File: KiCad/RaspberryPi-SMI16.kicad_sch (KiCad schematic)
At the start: 11 parts, among them J1 Screw_Terminal_01x02, U1 RASPBERRYPI_GPIO_40, U2 RFID-RC522

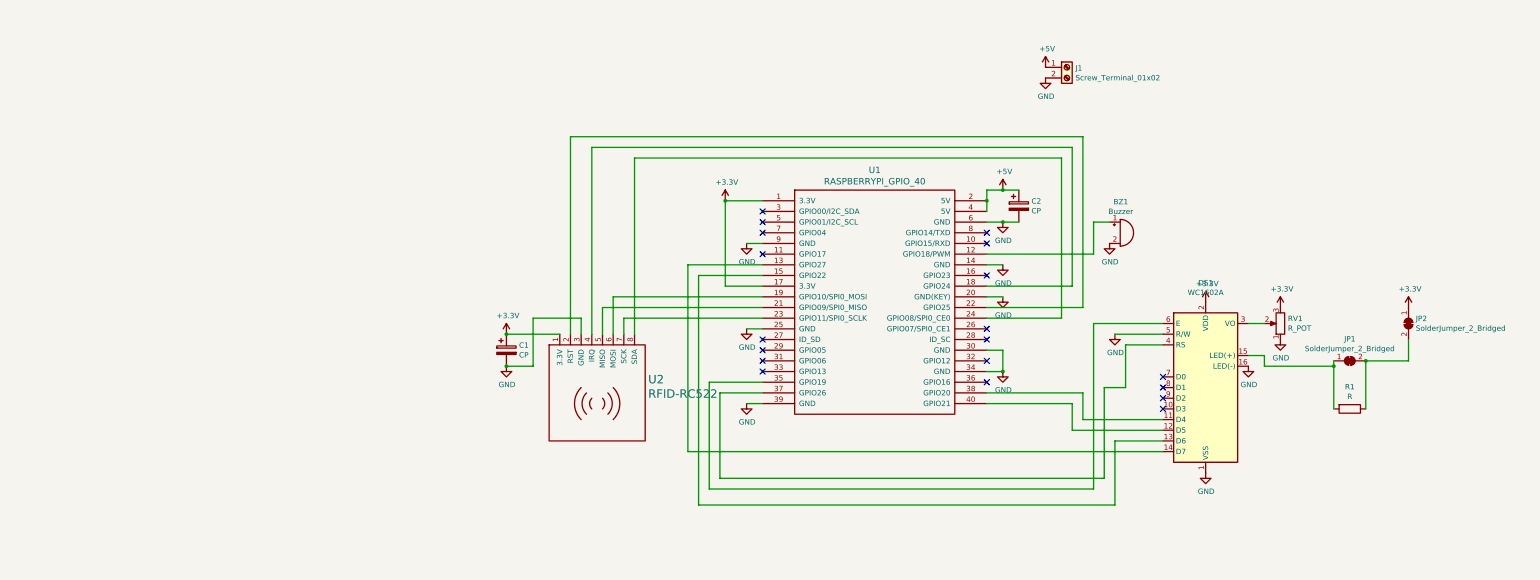
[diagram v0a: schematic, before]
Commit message: SMI HAT PCB create
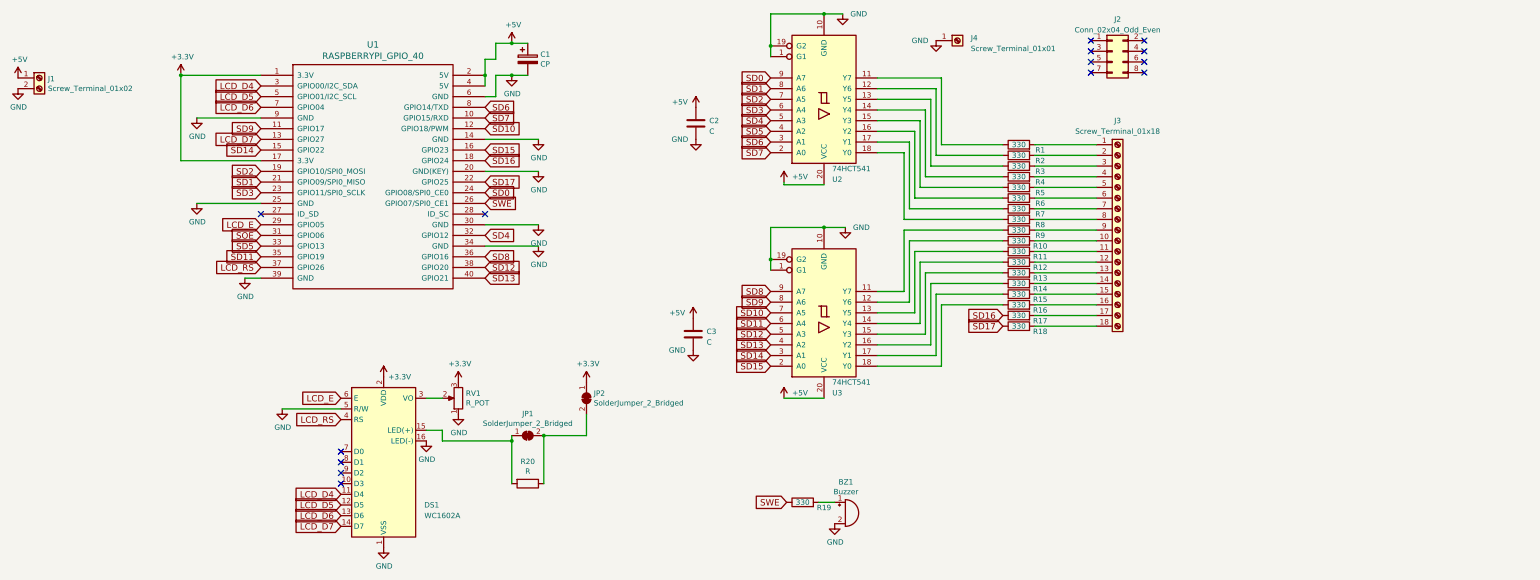
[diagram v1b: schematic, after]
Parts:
- removed C1: CP, Capacitor_THT:CP_Radial_D8.0mm_P3.50mm, symbol RaspberryPi-SMI16-rescue:CP-Device
- removed U2: RFID-RC522, library:RFID-RC522, symbol RaspberryPi-SMI16-rescue:RFID-RC522-nanbuwks
- added C2, C3: C, Capacitor_SMD:C_0603_1608Metric, symbol Device:C
- added J2: Conn_02x04_Odd_Even, MountingHole:MountingHole_3.2mm_M3, symbol Connector_Generic:Conn_02x04_Odd_Even
- added J3: Screw_Terminal_01x18, Connector_PinHeader_2.54mm:PinHeader_1x18_P2.54mm_Vertical, symbol Connector:Screw_Terminal_01x18
- added J4: Screw_Terminal_01x01, Connector_PinHeader_2.54mm:PinHeader_1x01_P2.54mm_Vertical, symbol Connector:Screw_Terminal_01x01
- added R1, R10, R11, R12, R13, R14, R15, R16, R17, R18, R19, R2, R3, R4, R5, R6, R7, R8, R9: 330, Resistor_SMD:R_0603_1608Metric, symbol Device:R
- added U2: 74HCT541, Package_SO:SOIC-20W_7.5x12.8mm_P1.27mm, symbol 74xx:74HCT541
- added U3: 74HCT541, Package_SO:SOIC-20W_7.5x15.4mm_P1.27mm, symbol 74xx:74HCT541
- J1: footprint TerminalBlock:TerminalBlock_bornier-2_P5.08mm -> TerminalBlock_Phoenix:TerminalBlock_Phoenix_MKDS-1,5-2_1x02_P5.00mm_Horizontal
- renumbered C2 to C1, R1 to R20
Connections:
- net +5V: now also C2.1, C3.1, U2.20 (VCC), U3.20 (VCC)
- net GND: now also C2.2, C3.2, J4.1 (Pin_1), U2.1 (G1), U2.10 (GND), U2.19 (G2), U3.1 (G1), U3.10 (GND), U3.19 (G2)
- net SD17: now reaches U1.22 (GPIO25)
- net SD17: now also R18.1
- net SD16: now reaches U1.18 (GPIO24)
- net SD16: now also R17.1
- net SD1: now reaches U1.21 (GPIO09/SPI0_MISO)
- net SD1: now also U2.8 (A6)
- net SD2: now reaches U1.19 (GPIO10/SPI0_MOSI)
- net SD2: now also U2.7 (A5)
- net SD3: now reaches U1.23 (GPIO11/SPI0_SCLK)
- net SD3: now also U2.6 (A4)
- net SD0: now reaches U1.24 (GPIO08/SPI0_CE0)
- net SD0: now also U2.9 (A7)
- net LCD_D4: now reaches DS1.11 (D4)
- net LCD_D4: now also U1.3 (GPIO00/I2C_SDA); no longer U1.38 (GPIO20)
- net LCD_D5: now reaches DS1.12 (D5)
- net LCD_D5: now also U1.5 (GPIO01/I2C_SCL); no longer U1.40 (GPIO21)
- net LCD_D6: now reaches DS1.13 (D6)
- net LCD_D6: now also U1.7 (GPIO04); no longer U1.15 (GPIO22)
- net LCD_D7: now reaches DS1.14 (D7), U1.13 (GPIO27)
- net LCD_RS: now reaches DS1.4 (RS), U1.37 (GPIO26)
- net LCD_E: now reaches DS1.6 (E)
- net LCD_E: now also U1.29 (GPIO05); no longer U1.35 (GPIO19)
- net at BZ1.1 (-): now also R19.2; no longer U1.12 (GPIO18/PWM)
- net SD7: now reaches U1.10 (GPIO15/RXD)
- net SD7: now also U2.2 (A0)
- net SD9: now reaches U1.11 (GPIO17)
- net SD9: now also U3.8 (A6)
- net SD15: now reaches U1.16 (GPIO23)
- net SD15: now also U3.2 (A0)
- net SWE: now reaches U1.26 (GPIO07/SPI0_CE1)
- net SWE: now also R19.1
- net SOE: now reaches U1.31 (GPIO06)
- net SD4: now reaches U1.32 (GPIO12)
- net SD4: now also U2.5 (A3)
- net SD5: now reaches U1.33 (GPIO13)
- net SD5: now also U2.4 (A2)
- net SD8: now reaches U1.36 (GPIO16)
- net SD8: now also U3.9 (A7)
- net SD6: now reaches U1.8 (GPIO14/TXD)
- net SD6: now also U2.3 (A1)
- new net: R16.1, U3.18 (Y0)
- new net: J3.16 (Pin_16), R16.2
- new net: R14.1, U3.16 (Y2)
- new net: J3.14 (Pin_14), R14.2
- new net: J3.17 (Pin_17), R17.2
- new net: R4.1, U2.14 (Y4)
- new net: J3.4 (Pin_4), R4.2
- new net: R6.1, U2.16 (Y2)
- new net: J3.6 (Pin_6), R6.2
- new net: R10.1, U3.12 (Y6)
- new net: J3.10 (Pin_10), R10.2
- new net: R12.1, U3.14 (Y4)
- new net: J3.12 (Pin_12), R12.2
- new net: R9.1, U3.11 (Y7)
- new net: J3.9 (Pin_9), R9.2
- new net: R11.1, U3.13 (Y5)
- new net: J3.11 (Pin_11), R11.2
- new net: R5.1, U2.15 (Y3)
- new net: J3.5 (Pin_5), R5.2
- new net: J3.1 (Pin_1), R1.2
- new net: J3.13 (Pin_13), R13.2
- new net: J3.15 (Pin_15), R15.2
- new net: J3.18 (Pin_18), R18.2
- new net: J3.2 (Pin_2), R2.2
- new net: J3.3 (Pin_3), R3.2
- new net: J3.7 (Pin_7), R7.2
- new net: J3.8 (Pin_8), R8.2
- new net: R2.1, U2.12 (Y6)
- new net: R7.1, U2.17 (Y1)
- new net: R15.1, U3.17 (Y1)
- new net: R13.1, U3.15 (Y3)
- new net: R8.1, U2.18 (Y0)
- new net: R3.1, U2.13 (Y5)
- new net: R1.1, U2.11 (Y7)
- new net SD10: U1.12 (GPIO18/PWM), U3.7 (A5)
- new net SD11: U1.35 (GPIO19), U3.6 (A4)
- new net SD12: U1.38 (GPIO20), U3.5 (A3)
- new net SD13: U1.40 (GPIO21), U3.4 (A2)
- new net SD14: U1.15 (GPIO22), U3.3 (A1)
- no-connect marks 19 -> 14
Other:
- moved on the sheet: BZ1, C1, DS1, J1, JP1, JP2, R20, RV1, U1
